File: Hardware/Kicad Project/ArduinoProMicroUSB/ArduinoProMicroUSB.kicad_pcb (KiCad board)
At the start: 4 copper layers, 32 x 26.4 mm, 41 parts, among them J1 Battery, J3 Display FPC, Q1 MMBT3904, U1 RV-3028-C7, U2 MIC5219, U3 USB-AB, U5 ATMEGA32U4QFN, Y1 16MHz

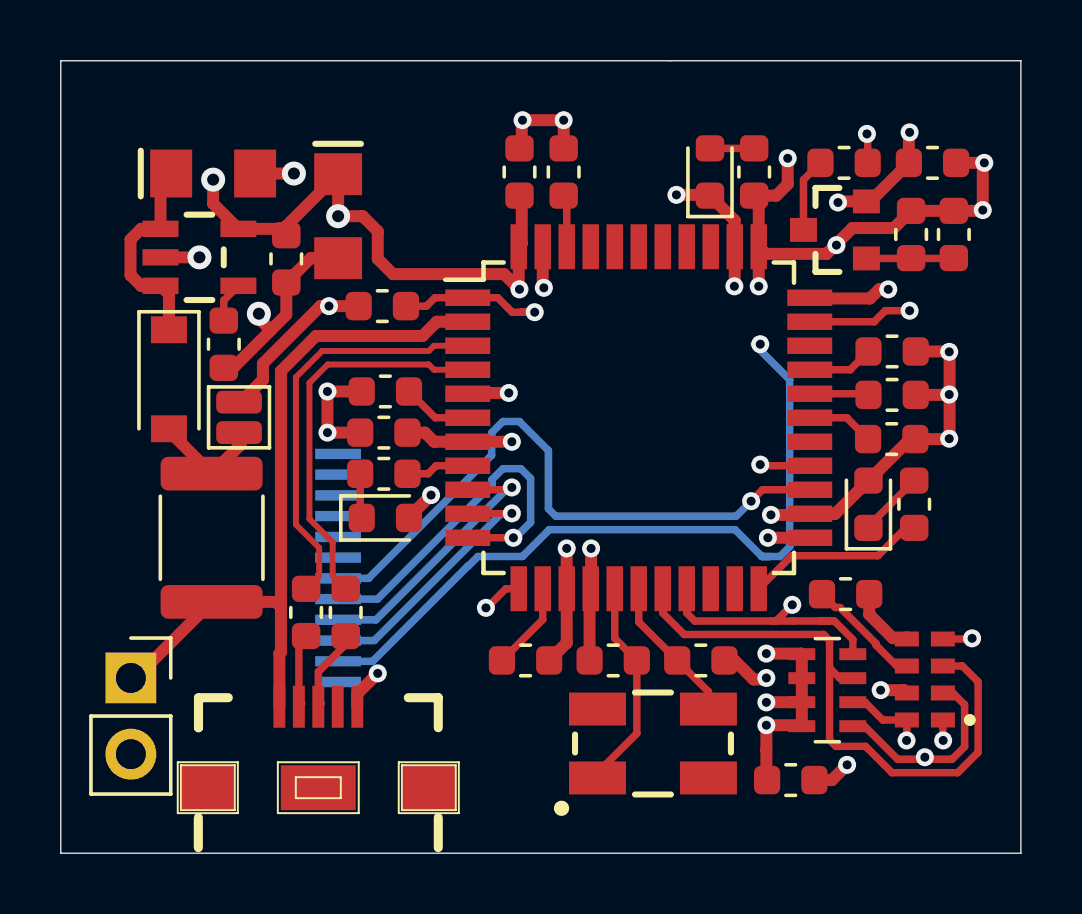
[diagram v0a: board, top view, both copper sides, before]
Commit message: rev 0.1
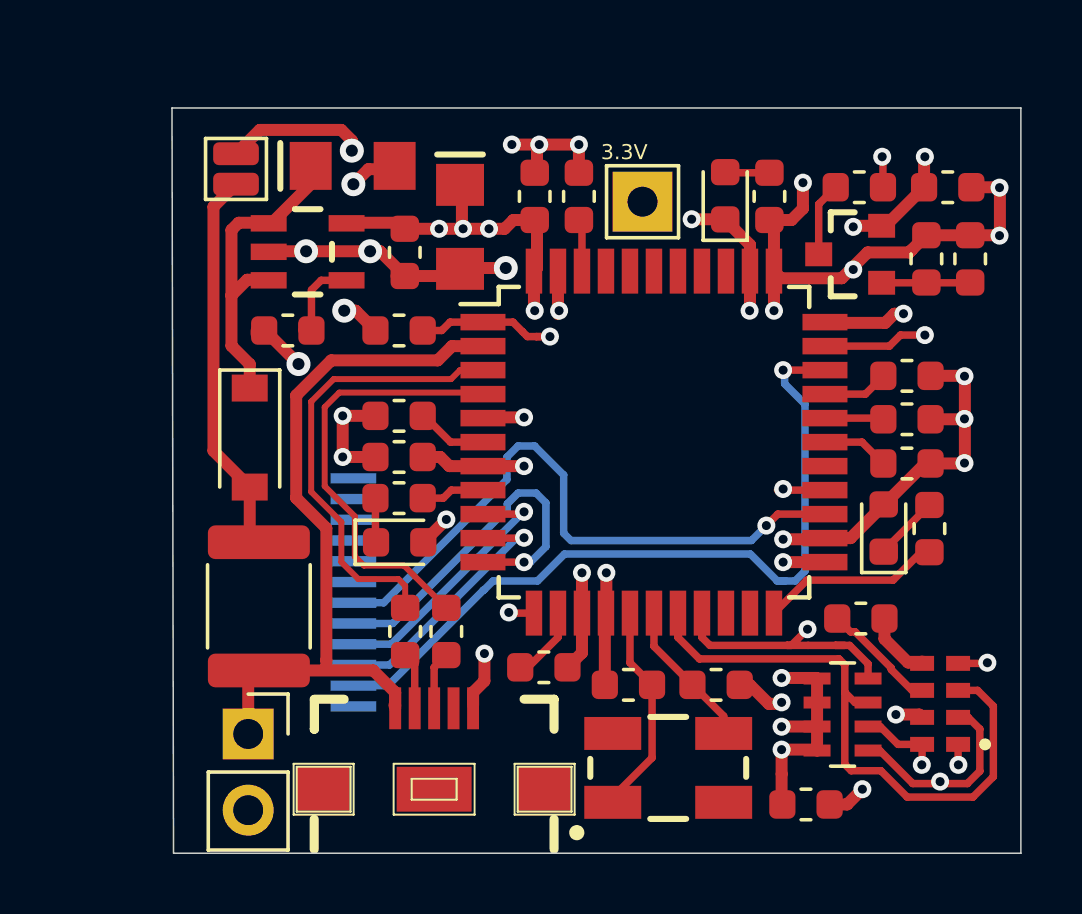
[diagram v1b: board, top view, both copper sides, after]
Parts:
- added 3.3V: TestPoint_THTPad_2.0x2.0mm_Drill1.0mm, TestPoint:TestPoint_THTPad_2.0x2.0mm_Drill1.0mm, F.Cu at (144.9, 77.9)
- moved SJ1 8.28 mm to (128.8, 77.3)
- moved C1 4.66 mm to (135.2, 76.7)
- moved J1 4.33 mm to (131.7, 95.6)
- moved C2 4.08 mm to (138.8, 78.7)
- moved C4 3.96 mm to (136.9, 79.5)
- moved U3 3.86 mm to (137.9, 97.4)
- moved U2 3.61 mm to (133.7, 79.5)
- moved R7 3.41 mm to (138.3, 92.2)
- moved R5 3.36 mm to (137.0, 92.2)
- moved D1 3.32 mm to (131.8, 85.7)
- moved F1 2.78 mm to (132.1, 91.3)
- moved C13 2.18 mm to (133.0, 82.1), turned to 180 degrees
- moved R12 0.99 mm to (136.8, 82.1)
- moved R3 0.98 mm to (155.8, 79.8)
- moved C8 0.96 mm to (150.3, 97.9)
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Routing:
- net Net-(D1-Pad2): track 3.86 -> 13.1 mm
- net 3.3V: track 66.3 -> 58.9 mm, vias 19 -> 21
- net GND: track 41.5 -> 46.9 mm, vias 19 -> 22
- net /RAW: track 7.05 -> 10.9 mm
- net /D+: track 13.0 -> 14.6 mm
- net Net-(C13-Pad1): track 1.36 -> 2.93 mm
- net /D-: track 13.7 -> 15.1 mm
- net /D5: track 25.0 -> 26.0 mm
- net Net-(R7-Pad2): track 2.88 -> 1.94 mm
- net Net-(R5-Pad2): track 2.60 -> 1.90 mm
- net Net-(R4-Pad2): track 2.99 -> 2.48 mm
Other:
- board size 32 x 26.4 mm -> 28.3 x 24.8 mm
